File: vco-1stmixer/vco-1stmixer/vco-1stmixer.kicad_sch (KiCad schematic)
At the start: 48 parts, among them J101 VCO Control In, J102 1st IF Out, J103 VCO Sample, J104 RF In, J105 Conn_01x02, U101 POS-200, U102 MAV-11, U103 MAV-11, U104 TUF-1H+

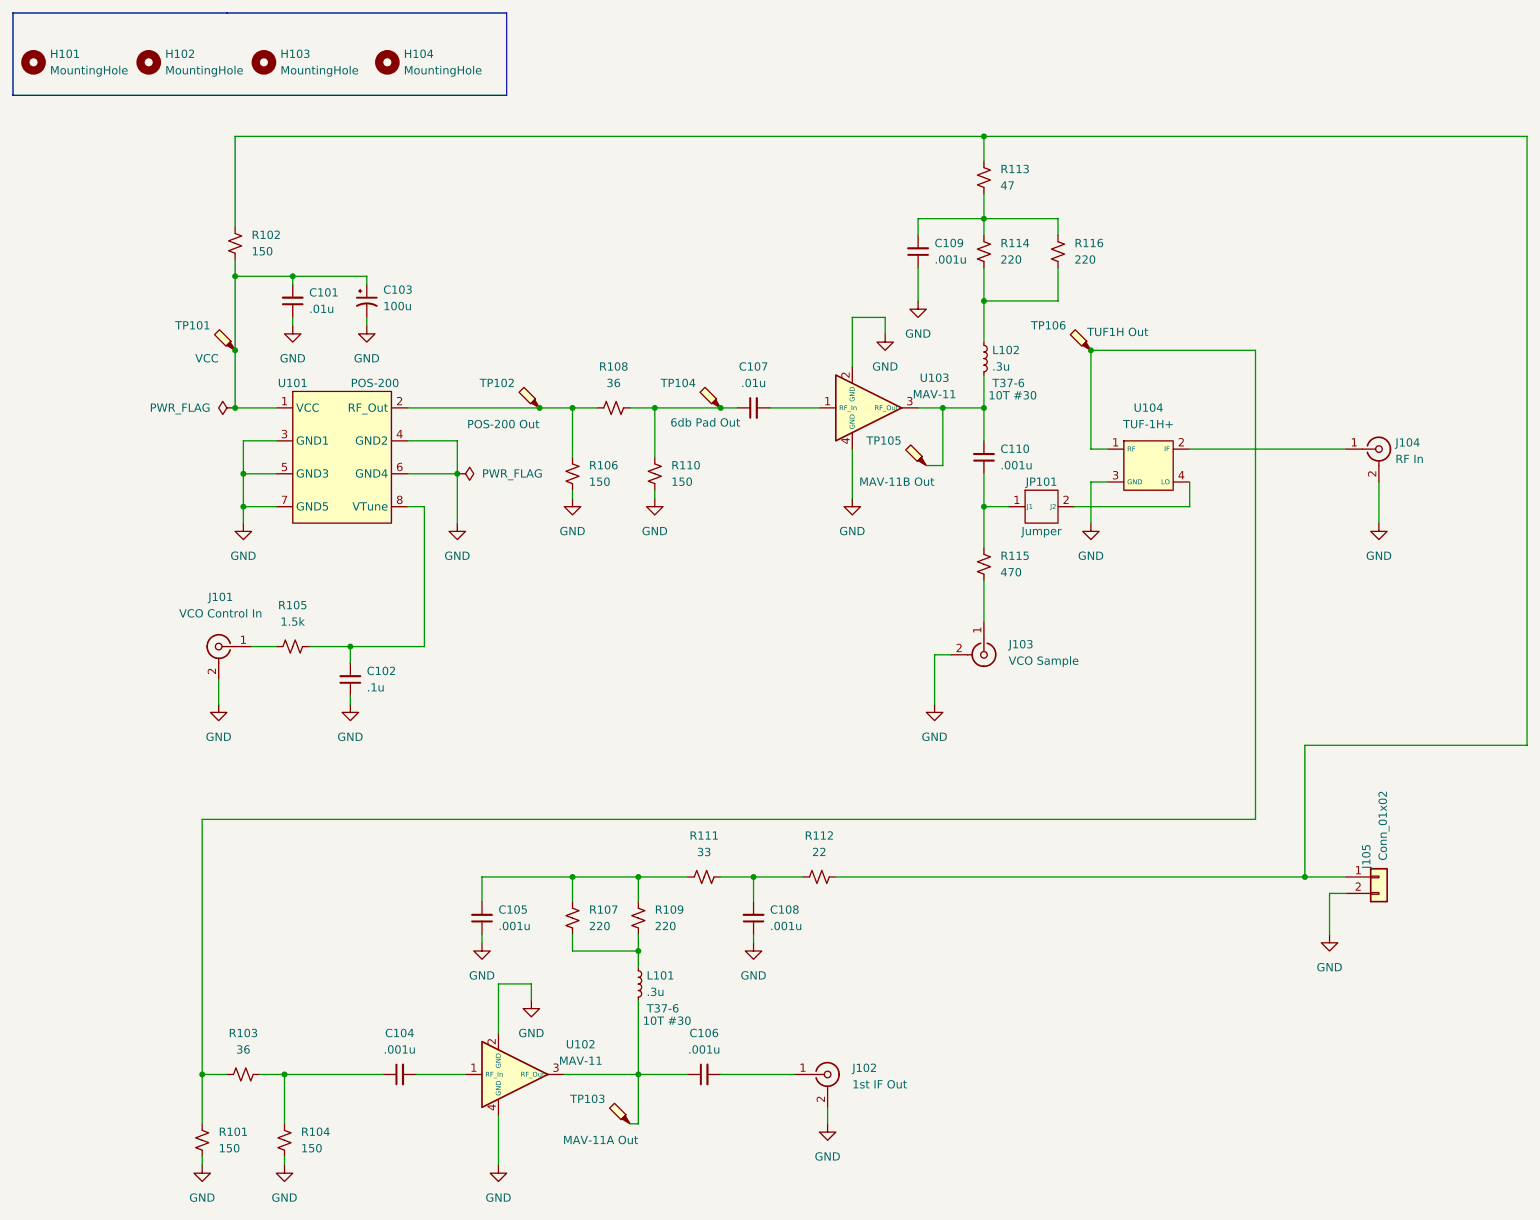
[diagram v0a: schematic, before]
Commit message: v7 conversion
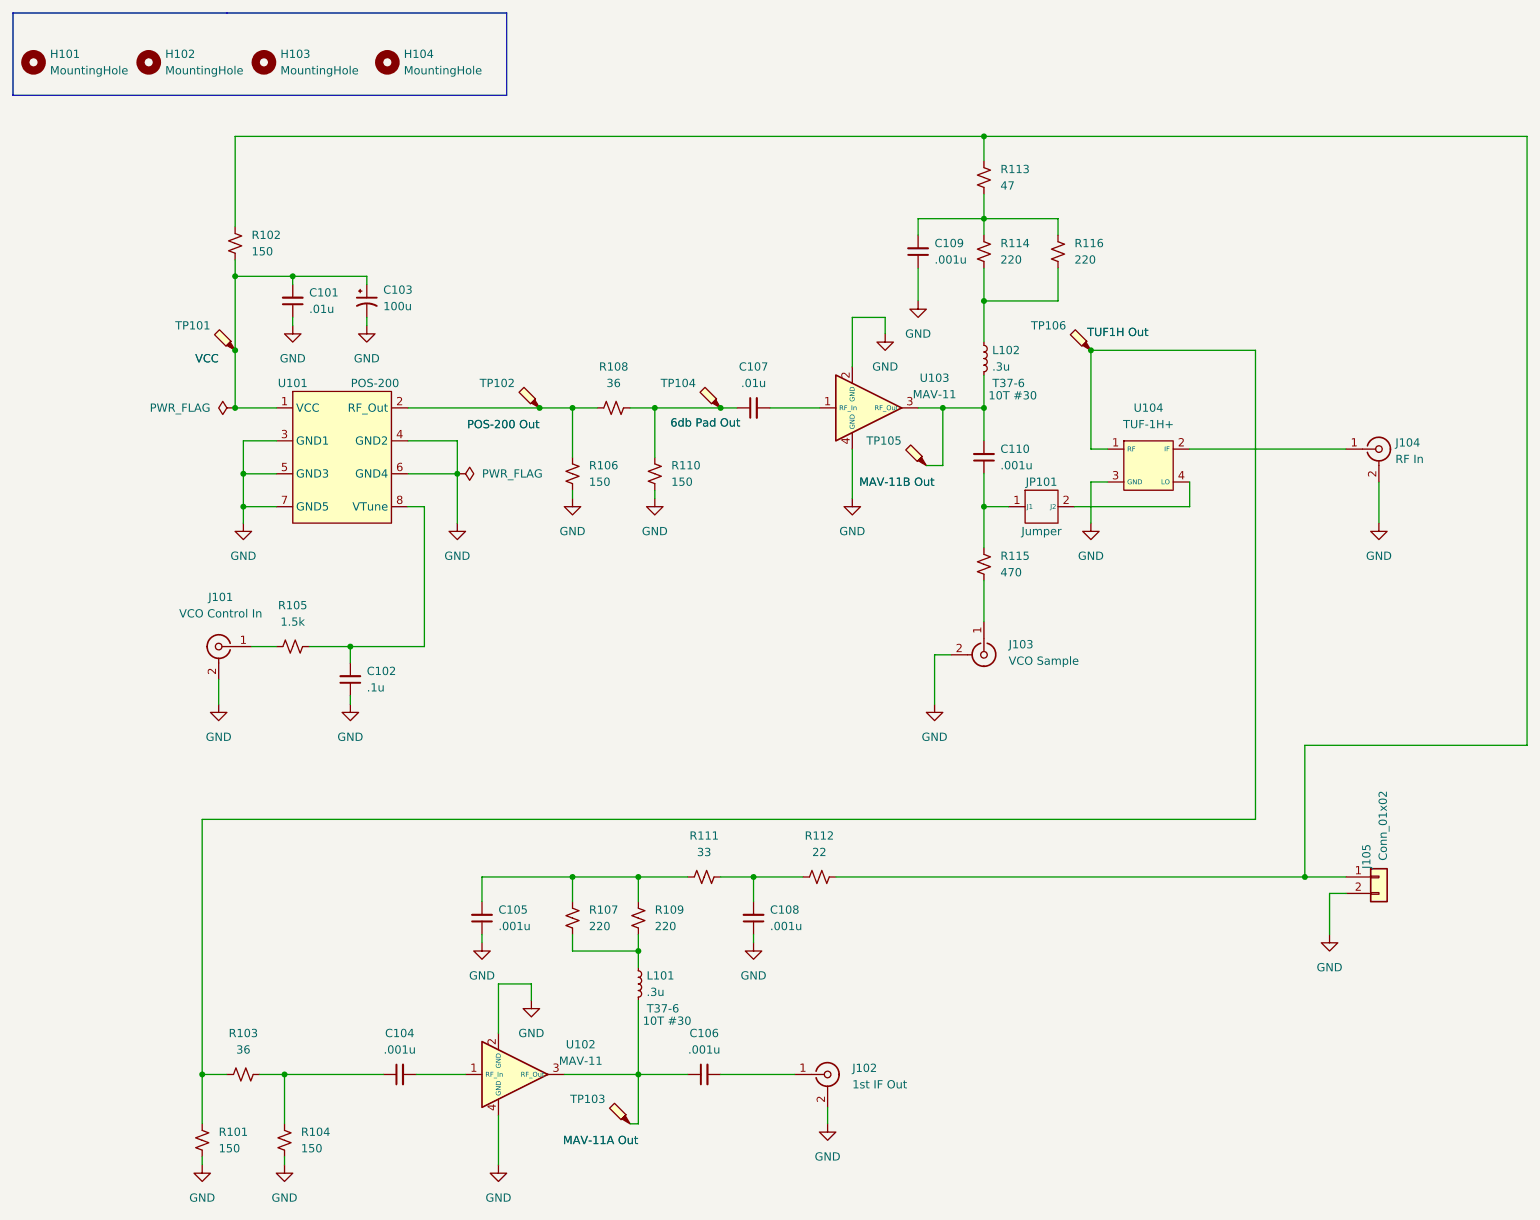
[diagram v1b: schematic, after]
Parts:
- J105: Spice_Model Conn_01x02 -> (none); Spice_Netlist_Enabled N -> (none); Spice_Primitive J -> (none)
- JP101: Spice_Model 22284028 -> (none); Spice_Netlist_Enabled N -> (none); Spice_Primitive J -> (none)
- TP101: value VCC -> ${SIM.PARAMS}; Spice_Netlist_Enabled N -> (none)
- TP102: value POS-200 Out -> ${SIM.PARAMS}; Spice_Netlist_Enabled N -> (none)
- TP103: value MAV-11A Out -> ${SIM.PARAMS}; Spice_Netlist_Enabled N -> (none)
- TP104: value 6db Pad Out -> ${SIM.PARAMS}; Spice_Netlist_Enabled N -> (none)
- TP105: value MAV-11B Out -> ${SIM.PARAMS}; Spice_Netlist_Enabled N -> (none)
- TP106: value TUF1H Out -> ${SIM.PARAMS}; Spice_Netlist_Enabled N -> (none)
